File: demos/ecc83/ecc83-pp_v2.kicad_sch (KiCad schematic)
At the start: 15 parts, among them P1 IN, P2 OUT, P3 POWER, P4 CONN_2, P5 CONN_1, P6 CONN_1, P7 CONN_1, P8 CONN_1, U1 ECC83

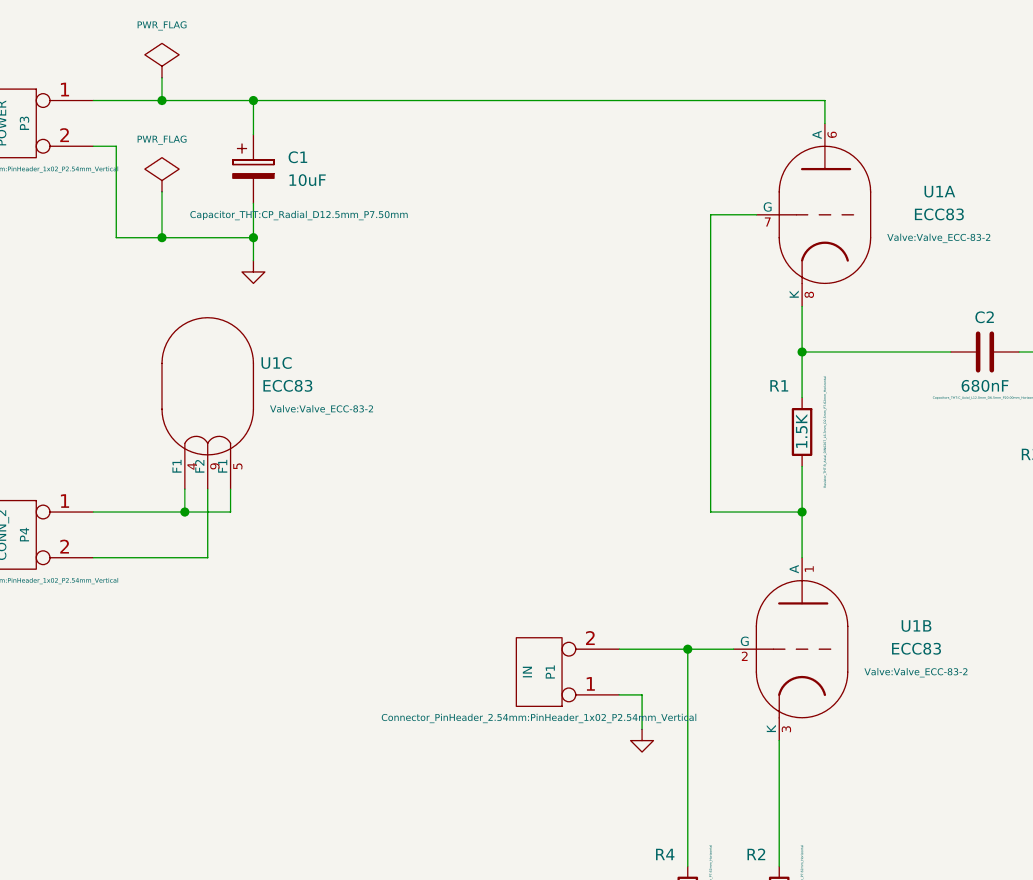
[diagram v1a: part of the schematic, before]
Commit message: Demos update
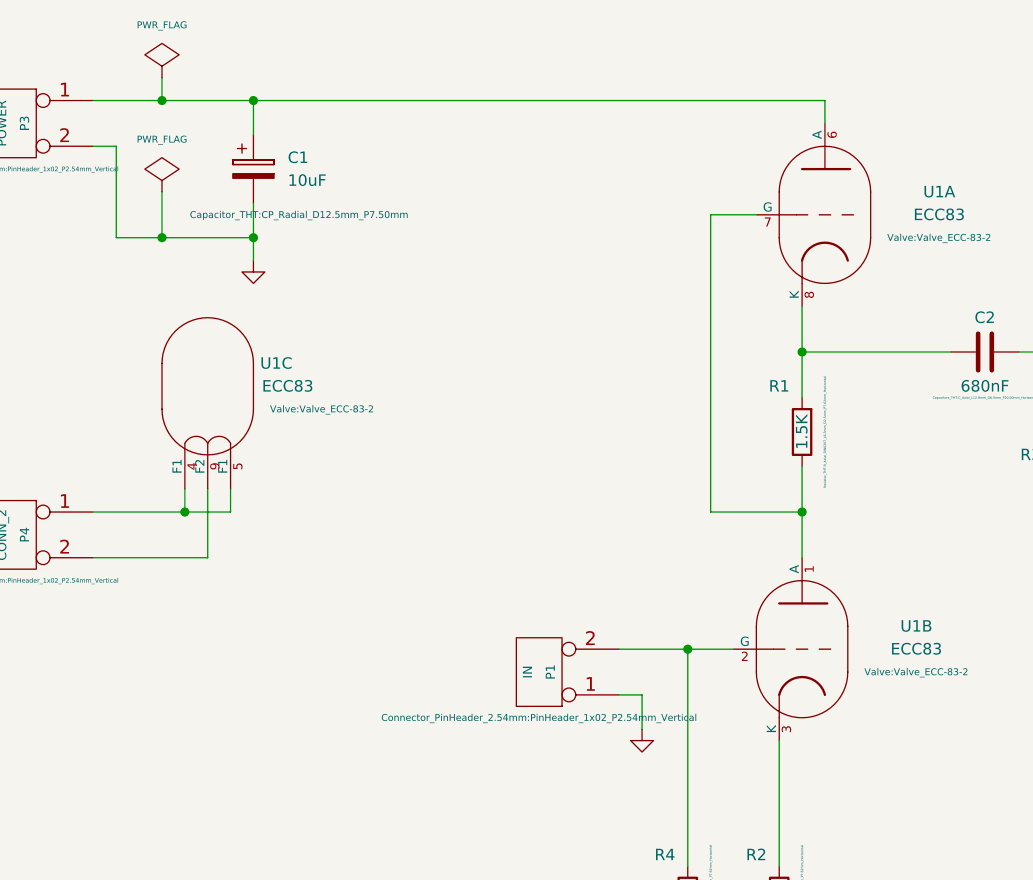
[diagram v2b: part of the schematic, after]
